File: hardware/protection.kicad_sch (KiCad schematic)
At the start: 3 parts

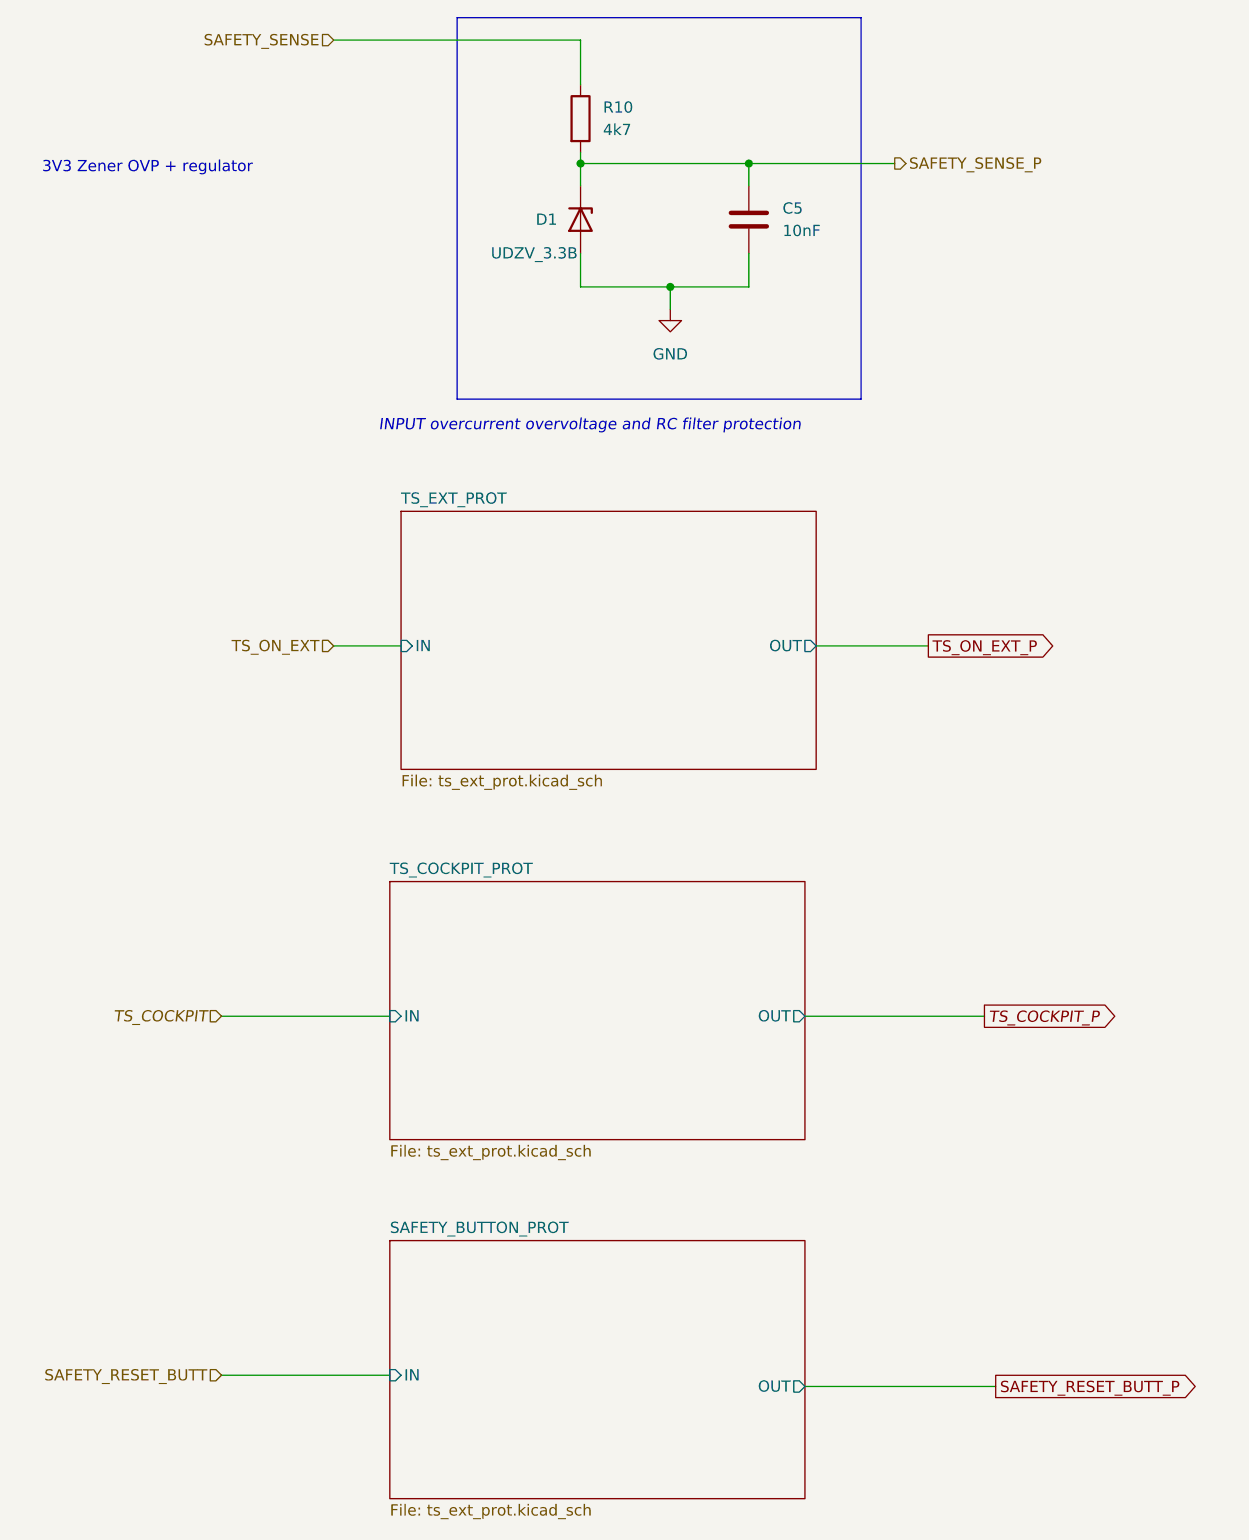
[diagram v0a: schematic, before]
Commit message: changed pcb version
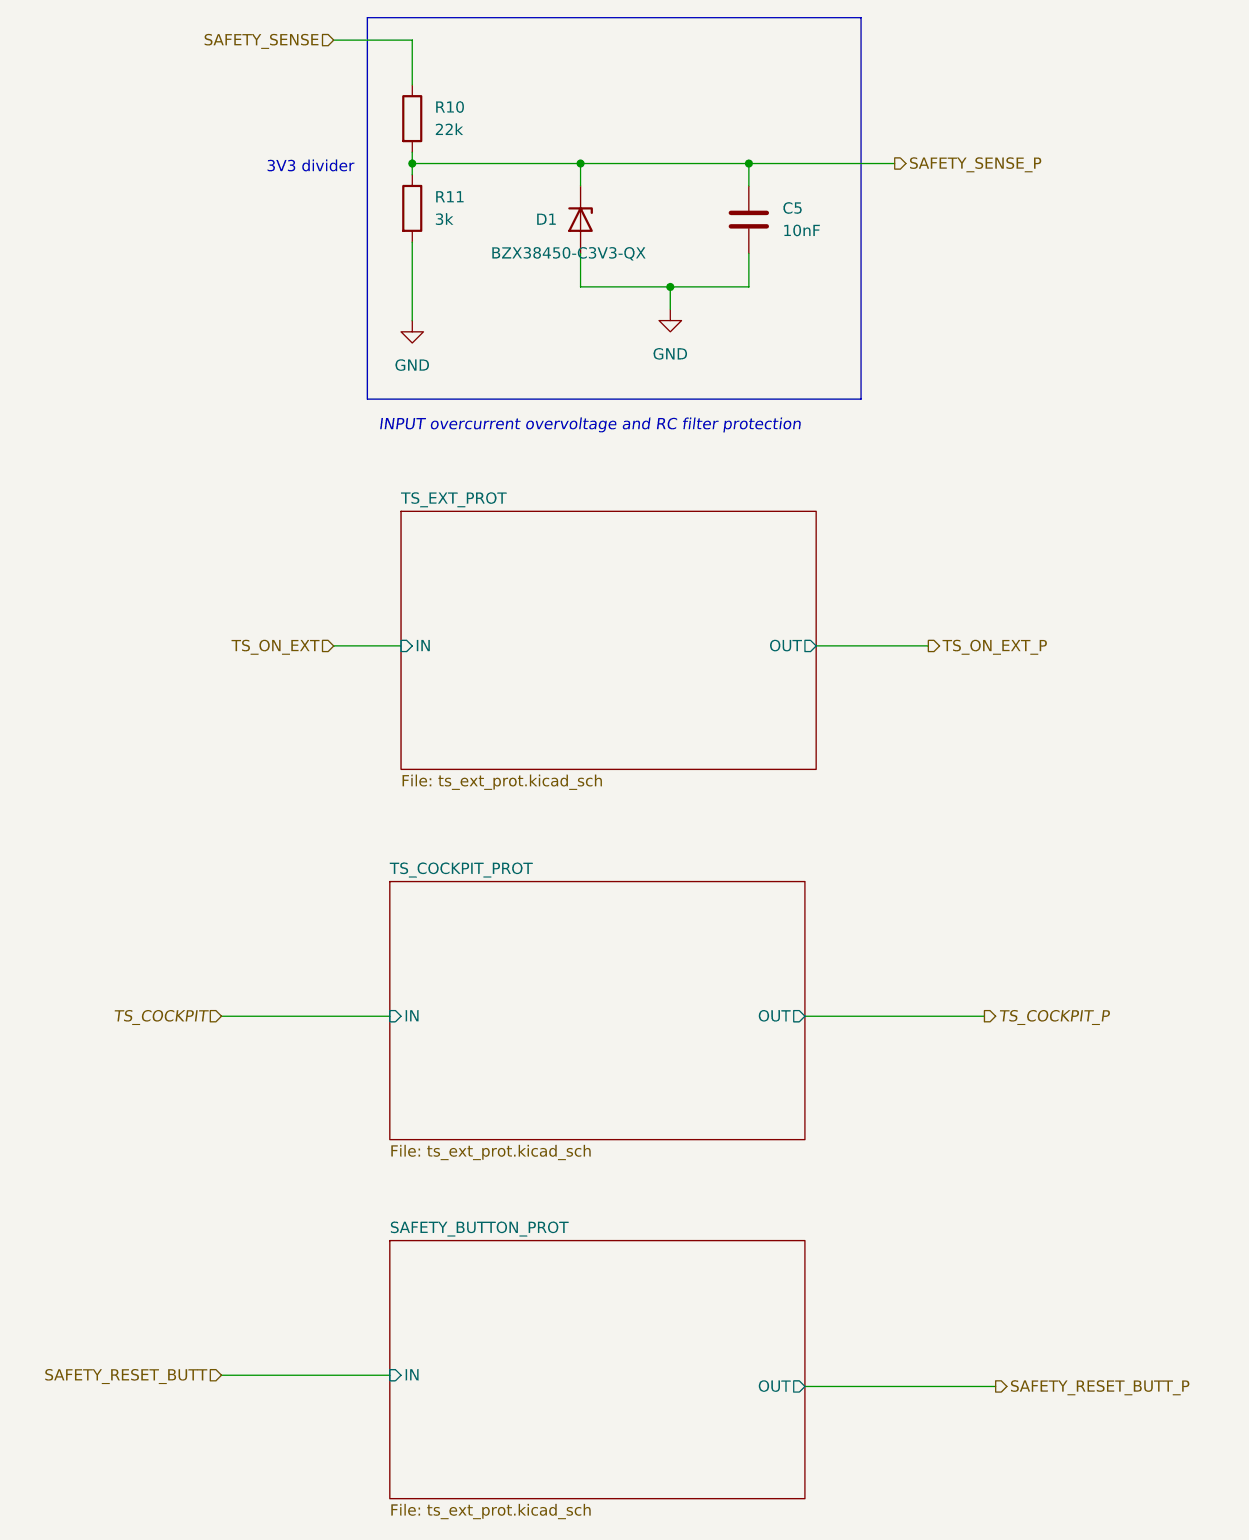
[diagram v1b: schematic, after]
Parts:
- added R11: 3k, Resistor_SMD:R_0603_1608Metric_Pad0.98x0.95mm_HandSolder, symbol Device:R
- D1: value UDZV_3.3B -> BZX38450-C3V3-QX
- R10: value 4k7 -> 22k
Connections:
- net GND: now also R11.2
- net SAFETY_SENSE_P: now also R11.1
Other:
- note added: "3V3 divider"
- note removed: "3V3 Zener OVP + regulator"
- moved on the sheet: R10
